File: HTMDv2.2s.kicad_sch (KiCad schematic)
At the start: 94 parts, among them IC1 TJA1441AT_0Z, IC2 A3921KLPTR-T, IC3 TMP275AQDGKRQ1, J1 Conn_01x04, J10 Conn_01x02, J11 Conn_01x02, J2 Conn_01x04, J3 Conn_01x06, J4 Conn_01x01, J5 Conn_01x01_Pin, J6 Conn_01x02_Pin, J7 Conn_01x01_Pin, J8 Conn_01x01, J9 Conn_01x04_Pin, SW2 SW_Push, SW3 SW_Push, U1 ADP3338AKCZ-3.3, U13 SQJ180EP-T1_GE3, U14 SQJ180EP-T1_GE3, U15 SQJ180EP-T1_GE3, U16 SQJ180EP-T1_GE3, U2 STM32G431CBUx, U3 ISO6741FDWR, U4 CZ3A07, U5 MCP3421A0T-ECH

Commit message: update PCB
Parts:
- IC1: footprint (none) -> 0-Myparts:SOIC127P600X175-8N
- IC3: footprint 0_Mylib:SOP65P490X110-8N -> 0_Mylib:TMP275AQDGKRQ1
- RV1, RV2: footprint Resistor_SMD:R_0603_1608Metric_Pad0.98x0.95mm_HandSolder -> 0-Myparts:TSR-3296
- U1: footprint (none) -> 0-Myparts:SOT230P700X180-4N
- U4: footprint 0_Mylib:CZ3A07 -> 0-Myparts:CZ3AG6
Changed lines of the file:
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@@
       (effects (font (size 1.27 1.27)) (justify right))
     )
-    (property "Footprint" "Resistor_SMD:R_0603_1608Metric_Pad0.98x0.95mm_HandSolder" (at 284.226 195.326 0)
+    (property "Footprint" "0-Myparts:TSR-3296" (at 284.226 195.326 0)
       (effects (font (size 1.27 1.27)) hide)
     )
@@
       (effects (font (size 1.27 1.27)))
     )
-    (property "Footprint" "" (at 102.235 41.783 0)
+    (property "Footprint" "0-Myparts:SOT230P700X180-4N" (at 102.235 41.783 0)
       (effects (font (size 1.27 1.27)) (justify bottom) hide)
     )
@@
       (effects (font (size 1.27 1.27)))
     )
-    (property "Footprint" "0_Mylib:SOP65P490X110-8N" (at 286.258 352.349 0)
+    (property "Footprint" "0_Mylib:TMP275AQDGKRQ1" (at 286.258 352.349 0)
       (effects (font (size 1.27 1.27)) (justify left top) hide)
     )
@@
       (effects (font (size 1.27 1.27)))
     )
-    (property "Footprint" "" (at 68.961 244.094 0)
+    (property "Footprint" "0-Myparts:SOIC127P600X175-8N" (at 68.961 244.094 0)
       (effects (font (size 1.27 1.27)) (justify left) hide)
     )
@@
       (effects (font (size 1.27 1.27)) (justify right))
     )
-    (property "Footprint" "Resistor_SMD:R_0603_1608Metric_Pad0.98x0.95mm_HandSolder" (at 312.42 195.199 0)
+    (property "Footprint" "0-Myparts:TSR-3296" (at 312.42 195.199 0)
       (effects (font (size 1.27 1.27)) hide)
     )
@@
       (effects (font (size 1.27 1.27)))
     )
-    (property "Footprint" "0_Mylib:CZ3A07" (at 197.612 283.769 0)
+    (property "Footprint" "0-Myparts:CZ3AG6" (at 197.612 283.769 0)
       (effects (font (size 1.27 1.27)) (justify left top) hide)
     )
@@
   )
   (symbol (lib_id "Analog_ADC:MCP3421A0T-ECH") (at 233.553 200.279 0) (unit 1)
-    (in_bom yes) (on_board yes) (dnp no) (fields_autoplaced)
+    (in_bom yes) (on_board yes) (dnp no)
     (property "Reference" "U5" (at 235.7471 189.23 0)
       (effects (font (size 1.27 1.27)) (justify left))

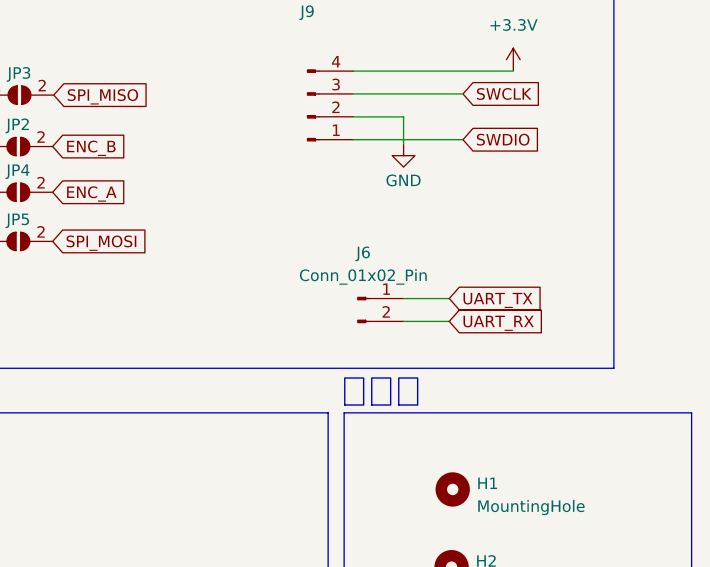
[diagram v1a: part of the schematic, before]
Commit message: update
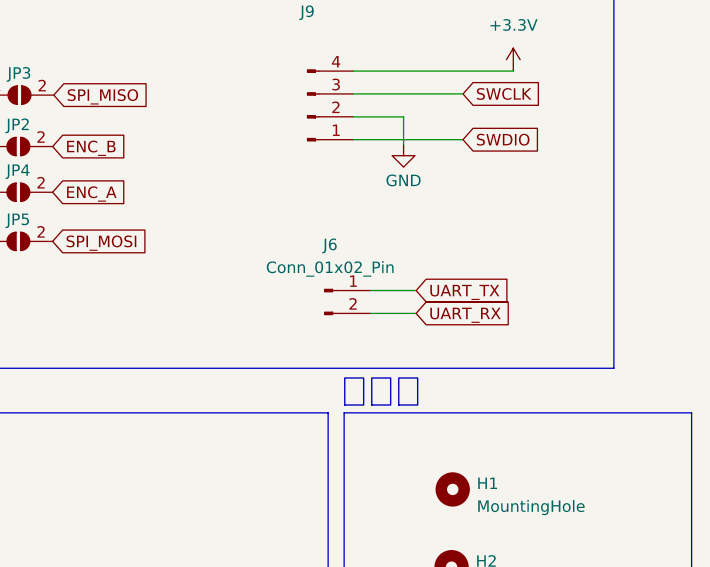
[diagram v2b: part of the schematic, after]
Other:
- moved on the sheet: J6
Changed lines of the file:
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@@
     (stroke (width 0) (type default))
   )
-  (wire (pts (xy 374.396 65.532) (xy 379.476 65.532))
+  (wire (pts (xy 370.713 64.643) (xy 375.793 64.643))
     (stroke (width 0) (type default))
   )
@@
     (stroke (width 0) (type default))
   )
-  (wire (pts (xy 374.396 62.992) (xy 379.476 62.992))
+  (wire (pts (xy 370.713 62.103) (xy 375.793 62.103))
     (stroke (width 0) (type default))
   )
@@
     )
   )
-  (global_label "UART_RX" (shape input) (at 379.476 65.532 0) (fields_autoplaced)
-    (effects (font (size 1.27 1.27)) (justify left))
-    (property "Intersheetrefs" "${INTERSHEET_REFS}" (at 390.565 65.532 0)
+  (global_label "UART_RX" (shape input) (at 375.793 64.643 0) (fields_autoplaced)
+    (effects (font (size 1.27 1.27)) (justify left))
+    (property "Intersheetrefs" "${INTERSHEET_REFS}" (at 386.882 64.643 0)
       (effects (font (size 1.27 1.27)) (justify left) hide)
     )
@@
     )
   )
-  (global_label "UART_TX" (shape input) (at 379.476 62.992 0) (fields_autoplaced)
-    (effects (font (size 1.27 1.27)) (justify left))
-    (property "Intersheetrefs" "${INTERSHEET_REFS}" (at 390.2626 62.992 0)
+  (global_label "UART_TX" (shape input) (at 375.793 62.103 0) (fields_autoplaced)
+    (effects (font (size 1.27 1.27)) (justify left))
+    (property "Intersheetrefs" "${INTERSHEET_REFS}" (at 386.5796 62.103 0)
       (effects (font (size 1.27 1.27)) (justify left) hide)
     )
@@
     )
   )
-  (symbol (lib_id "Connector:Conn_01x02_Pin") (at 369.316 62.992 0) (unit 1)
-    (in_bom yes) (on_board yes) (dnp no) (fields_autoplaced)
-    (property "Reference" "J6" (at 369.951 57.912 0)
-      (effects (font (size 1.27 1.27)))
-    )
-    (property "Value" "Conn_01x02_Pin" (at 369.951 60.452 0)
-      (effects (font (size 1.27 1.27)))
-    )
-    (property "Footprint" "Connector_PinHeader_2.54mm:PinHeader_1x02_P2.54mm_Horizontal" (at 369.316 62.992 0)
-      (effects (font (size 1.27 1.27)) hide)
-    )
-    (property "Datasheet" "~" (at 369.316 62.992 0)
-      (effects (font (size 1.27 1.27)) hide)
-    )
+  (symbol (lib_id "Connector:Conn_01x02_Pin") (at 365.633 62.103 0) (unit 1)
+    (in_bom yes) (on_board yes) (dnp no) (fields_autoplaced)
+    (property "Reference" "J6" (at 366.268 57.023 0)
+      (effects (font (size 1.27 1.27)))
+    )
+    (property "Value" "Conn_01x02_Pin" (at 366.268 59.563 0)
+      (effects (font (size 1.27 1.27)))
+    )
+    (property "Footprint" "Connector_PinHeader_2.54mm:PinHeader_1x02_P2.54mm_Horizontal" (at 365.633 62.103 0)
+      (effects (font (size 1.27 1.27)) hide)
+    )
+    (property "Datasheet" "~" (at 365.633 62.103 0)
+      (effects (font (size 1.27 1.27)) hide)
+    )
